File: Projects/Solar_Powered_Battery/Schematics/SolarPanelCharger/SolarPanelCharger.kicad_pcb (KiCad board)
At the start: 2 copper layers, 60 x 44 mm, 81 parts, among them J1 Conn_01x04_Female, J2 Conn_01x05_Female, J3 USB_B_Female, Q1 BC847, Q2 BC847, Q3 BC847, Q4 AO3401A, Q5 AO3401A, Q6 AO3400, Q7 AO3400, Q8 AO3401A, Q9 AO3401A, U1 LM358, U2 TL431DBZ, U3 TD1583, U4 TP4056, U5 MT3608

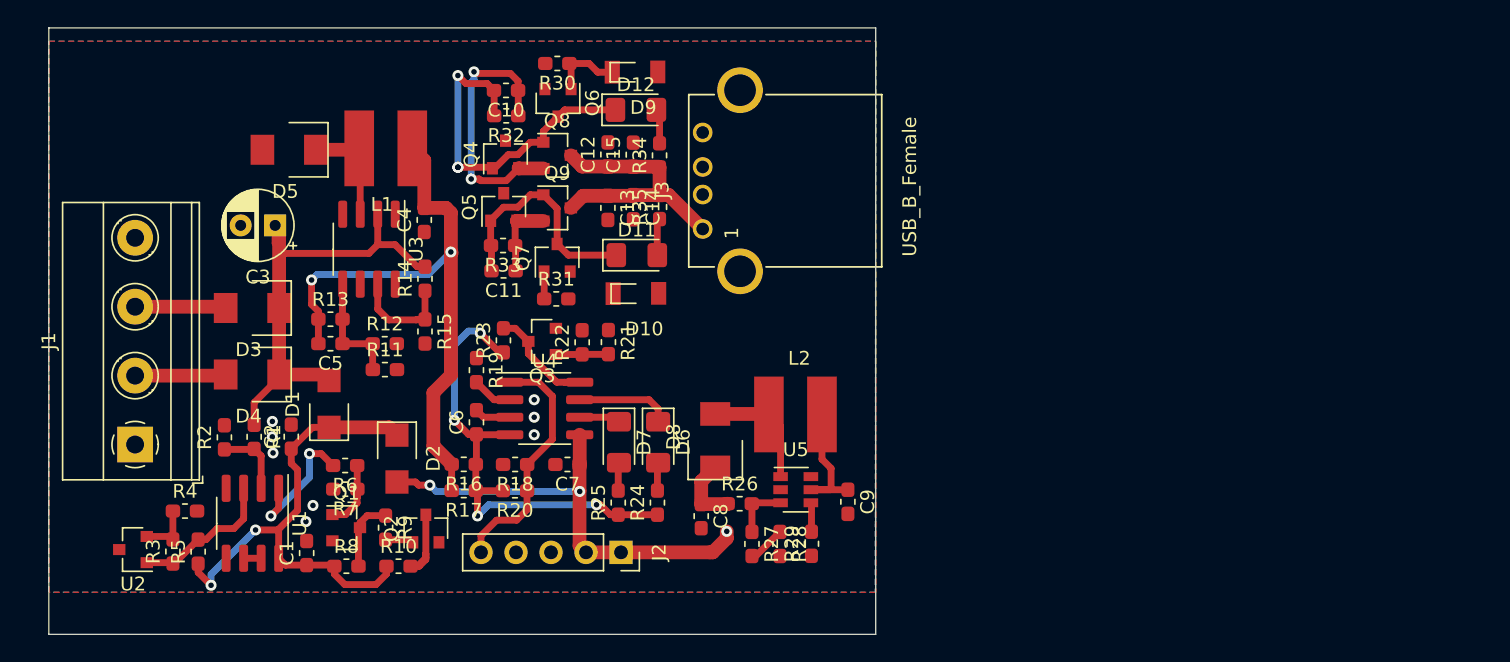
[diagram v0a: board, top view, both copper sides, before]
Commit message: pcb updated
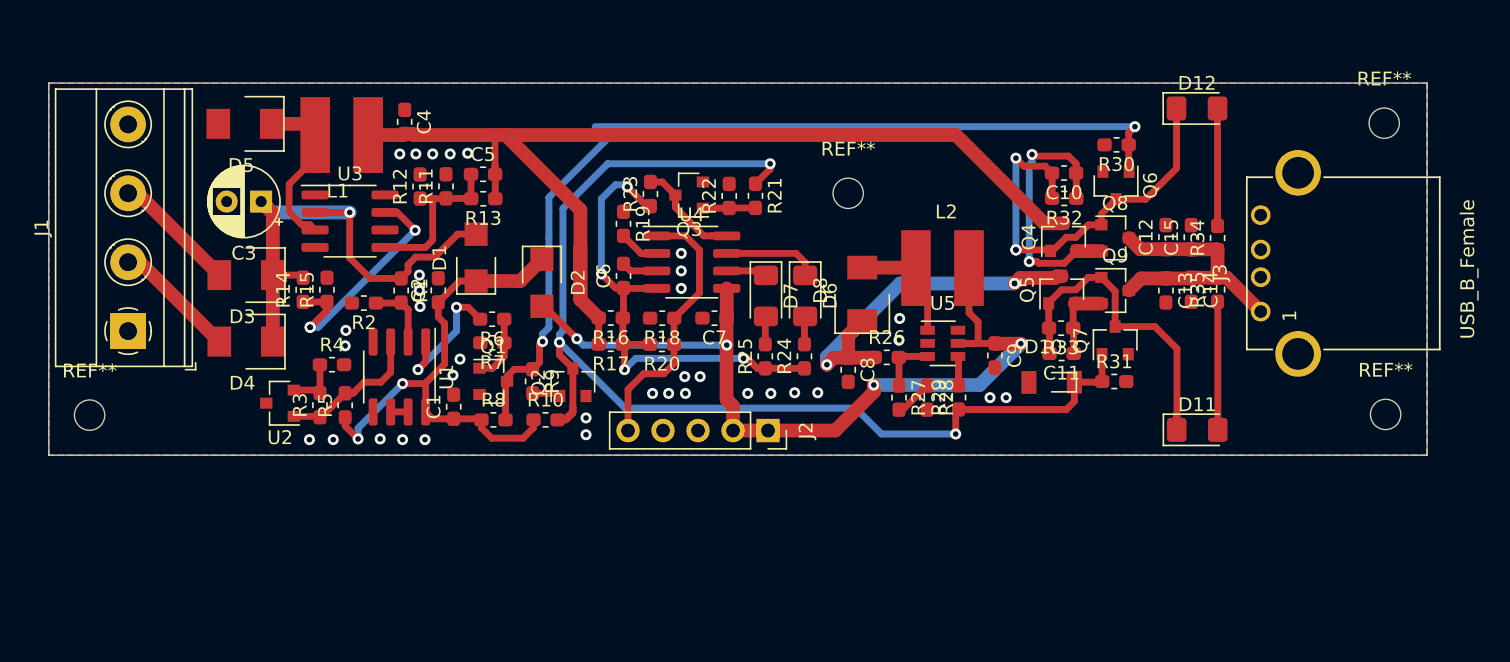
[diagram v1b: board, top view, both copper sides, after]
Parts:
- removed D9: 7V5, custom-footprints:LL34
- added REF**: MountingHole_2.2mm_M2, MountingHole:MountingHole_2.2mm_M2, F.Cu at (23.0, 44.1)
- added REF**: MountingHole_2.2mm_M2, MountingHole:MountingHole_2.2mm_M2, F.Cu at (117.0, 44.0)
- added REF**: MountingHole_2.2mm_M2, MountingHole:MountingHole_2.2mm_M2, F.Cu at (116.9, 22.9)
- added REF**: MountingHole_2.2mm_M2, MountingHole:MountingHole_2.2mm_M2, F.Cu at (78.0, 28.0)
- moved D11 42.6 mm to (103.3, 45.2)
- moved R30 41.0 mm to (97.5, 24.5)
- moved Q7 40.9 mm to (97.4, 38.7)
- moved Q8 40.9 mm to (97.4, 31.2)
- moved Q9 40.9 mm to (97.4, 35.1)
- moved R32 40.9 mm to (93.7, 28.4)
- moved R33 40.9 mm to (93.4, 37.8)
- moved C11 40.9 mm to (93.5, 39.6)
- moved C12 40.9 mm to (101.1, 31.2)
- moved C13 40.9 mm to (101.1, 35.1)
- moved J3 40.9 mm to (110.6, 33.1)
- moved Q5 40.9 mm to (93.5, 35.0)
- moved R31 40.9 mm to (97.3, 41.7)
- moved R34 40.9 mm to (104.8, 31.2)
- moved R35 40.9 mm to (104.8, 35.0)
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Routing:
- net /EN_BAT: track 7.43 -> 83.3 mm, vias 0 -> 3
- net /_EN_BAT: track 10.6 -> 68.1 mm, vias 0 -> 2
- net /Buck_5V0/BUCK_5V0: track 43.8 -> 79.6 mm, vias 2 -> 0
- net /BOOST_5V0/BOOST_OUT: track 5.01 -> 26.8 mm, vias 0 -> 3
- net /BOOST_5V0/BOOST_IN: track 43.3 -> 60.7 mm, vias 3 -> 4
- net /Buck_5V0/EN: track 7.65 -> 17.3 mm, vias 0 -> 3
- net Net-(D11-Pad2): track 2.69 -> 9.30 mm
- net Net-(C11-Pad2): track 16.9 -> 23.3 mm
- net Net-(D12-Pad2): track 2.52 -> 8.52 mm
- net Net-(C10-Pad2): track 25.3 -> 30.6 mm
- net Net-(D5-Pad1): track 7.99 -> 12.3 mm
- net Net-(C5-Pad1): track 8.40 -> 12.2 mm
- net Net-(D3-Pad2): track 6.61 -> 9.08 mm
- net Net-(D4-Pad2): track 6.60 -> 9.01 mm
- net /Buck_5V0/BUCK_IN: track 34.7 -> 36.8 mm, vias 0 -> 1
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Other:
- board size 60 x 44 mm -> 100 x 27 mm
